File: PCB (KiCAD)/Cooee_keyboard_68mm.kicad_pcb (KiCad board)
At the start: 2 copper layers, 67.9 x 51 mm, 99 parts, among them J1 Conn_01x15_Pin

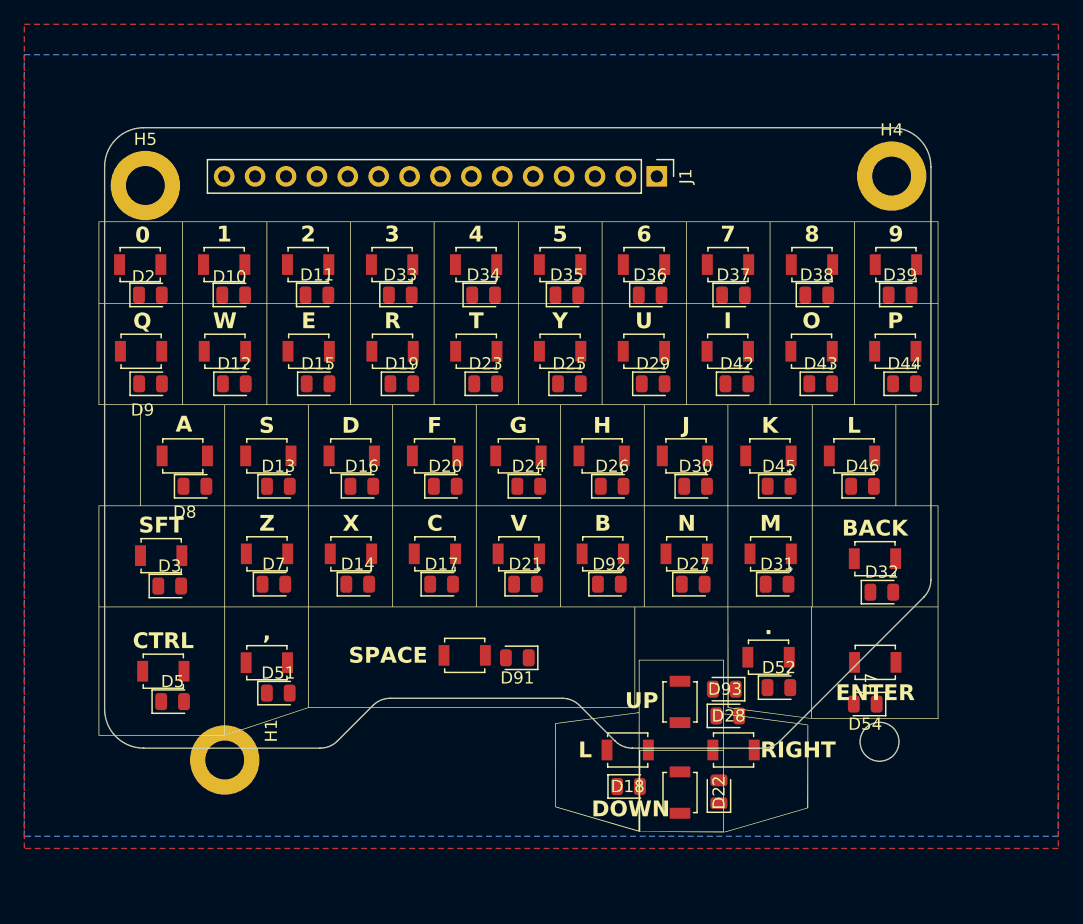
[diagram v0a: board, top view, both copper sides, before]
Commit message: finished routing new smaller keyboard
finished routing new smaller keyboard
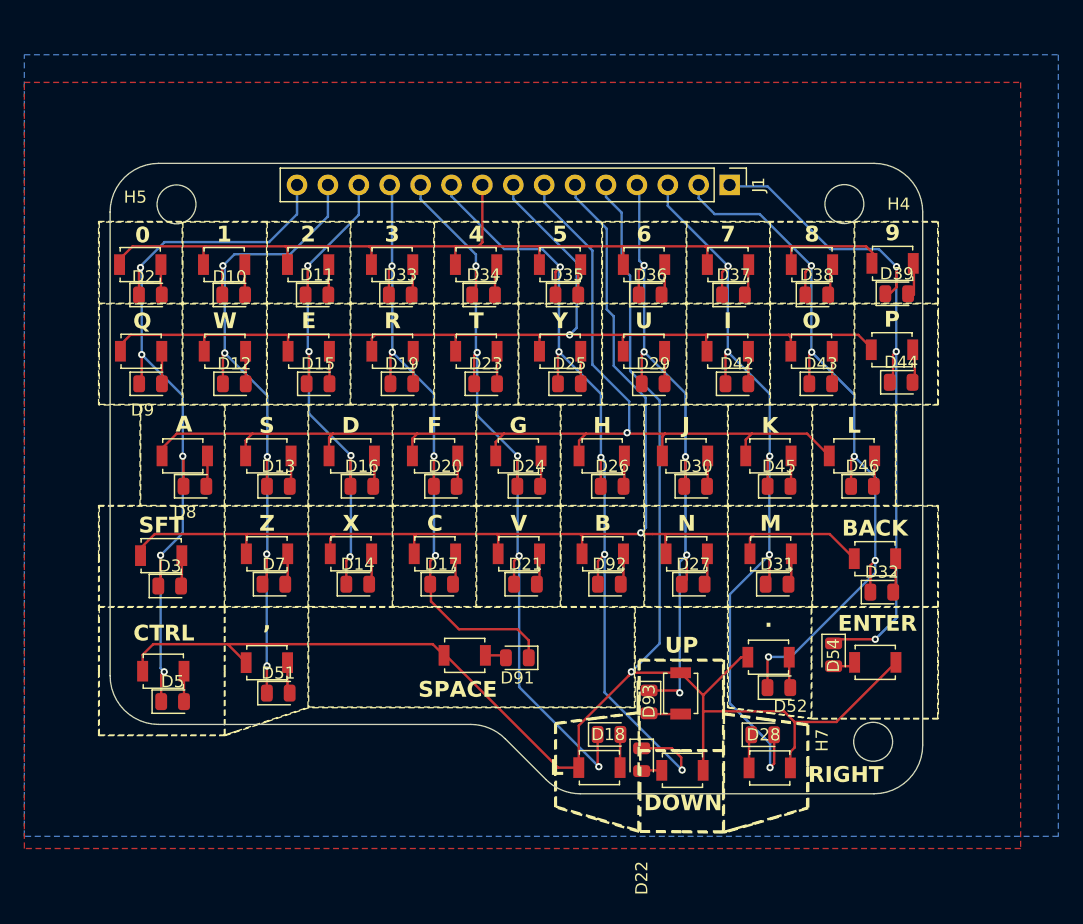
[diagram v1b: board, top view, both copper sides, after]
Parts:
- removed H1: MountingHole, MountingHole:MountingHole_3.2mm_M3_ISO7380_Pad
- H4, H5: footprint MountingHole:MountingHole_3.2mm_M3_ISO7380_Pad -> MountingHole:MountingHole_3.2mm_M3
- moved D22 6.88 mm to (160.5, 120.5), turned to -90 degrees
- moved D93 6.28 mm to (161.1, 115.7), turned to -90 degrees
- moved J1 6.03 mm to (167.7, 73.2)
- moved D54 4.81 mm to (176.3, 111.8), turned to -90 degrees
- moved D18 4.56 mm to (157.8, 118.4)
- moved H4 4.52 mm to (177.2, 74.8)
- moved SWe7 3.32 mm to (171.0, 121.1)
- moved D28 3.27 mm to (170.4, 118.4)
- moved SWe13 2.74 mm to (157.0, 121.1)
- moved H5 2.58 mm to (121.8, 74.8)
- moved SWe2 1.84 mm to (163.8, 121.3), turned to 180 degrees
- moved SWe88 0.70 mm to (163.7, 115.0)
- moved H7 0.53 mm to (179.5, 119.0)
- moved D44 0.30 mm to (181.8, 89.4)
- moved SWe37 0.30 mm to (181.1, 86.8)
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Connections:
- D14 pad 1: COL2 -> COL3
- D17 pad 1: COL3 -> COL4
- D21 pad 1: COL4 -> COL5
- D22 pad 1: COL5 -> COL6
- D27 pad 1: COL6 -> COL7
- D28 pad 2: COL7 -> COL8
- D31 pad 1: COL7 -> COL8
- D39 pad 1: COL9 -> COL10
- D44 pad 1: COL9 -> COL10
- D5 pad 1: COL2 -> COL1
- D51 pad 1: COL8 -> COL2
- D52 pad 1: COL8 -> COL9
- D54 pad 1: COL8 -> COL10
- D7 pad 1: COL1 -> COL2
- D92 pad 1: COL5 -> COL6
- D93 pad 1: COL6 -> COL7
- J1 pad 1: ROW6 -> COL10
- J1 pad 2: ROW5 -> COL9
- J1 pad 3: ROW4 -> COL8
- J1 pad 4: ROW3 -> COL7
- J1 pad 5: ROW2 -> ROW5
- J1 pad 6: ROW1 -> ROW4
- J1 pad 7: COL9 -> ROW3
- J1 pad 8: COL8 -> ROW2
- J1 pad 9: COL7 -> ROW1
- SWe17 pad 1: ROW5 -> ROW4
- SWe2 pad 1: ROW6 -> ROW5
- SWe24 pad 1: ROW5 -> ROW4
- SWe29 pad 1: ROW2 -> ROW1
- SWe36 pad 1: ROW3 -> ROW2
- SWe37 pad 1: ROW6 -> ROW2
- SWe39 pad 1: ROW4 -> ROW3
- SWe47 pad 1: ROW4 -> ROW5
- SWe50 pad 1: ROW6 -> ROW5
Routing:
- net ROW5: track 0.00 -> 136.3 mm, vias 0 -> 1
- net ROW4: track 0.00 -> 103.9 mm, vias 0 -> 1
- net ROW3: track 0.00 -> 94.2 mm, vias 0 -> 1
- net ROW2: track 0.00 -> 89.4 mm, vias 0 -> 1
- net ROW1: track 0.00 -> 82.2 mm
- net COL6: track 0.00 -> 72.7 mm, vias 0 -> 5
- net COL8: track 0.00 -> 67.3 mm, vias 0 -> 5
- net COL5: track 0.00 -> 66.8 mm, vias 0 -> 5
- net COL1: track 0.00 -> 65.2 mm, vias 0 -> 5
- net COL9: track 0.00 -> 64.9 mm, vias 0 -> 5
- net COL2: track 0.00 -> 59.6 mm, vias 0 -> 5
- net COL10: track 0.00 -> 57.0 mm, vias 0 -> 3
- net COL7: track 0.00 -> 56.6 mm, vias 0 -> 5
- net COL4: track 0.00 -> 54.4 mm, vias 0 -> 4
- net COL3: track 0.00 -> 43.9 mm, vias 0 -> 4
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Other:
- board size 67.9 x 51 mm -> 66.8 x 51.8 mm
